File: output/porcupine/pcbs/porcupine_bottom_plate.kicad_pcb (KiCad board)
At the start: 2 copper layers, 129.4 x 113.9 mm, 0 parts

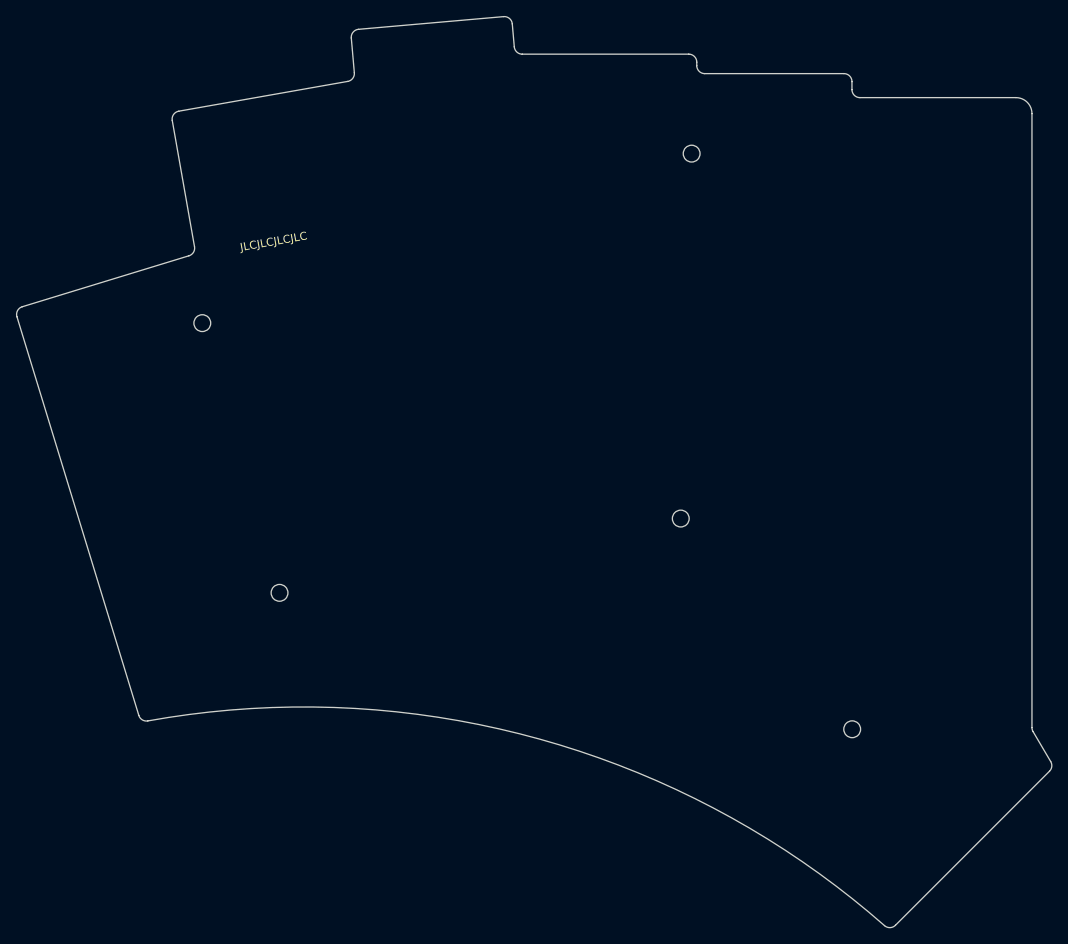
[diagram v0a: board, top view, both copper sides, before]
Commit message: Beschreibung deiner Änderungen
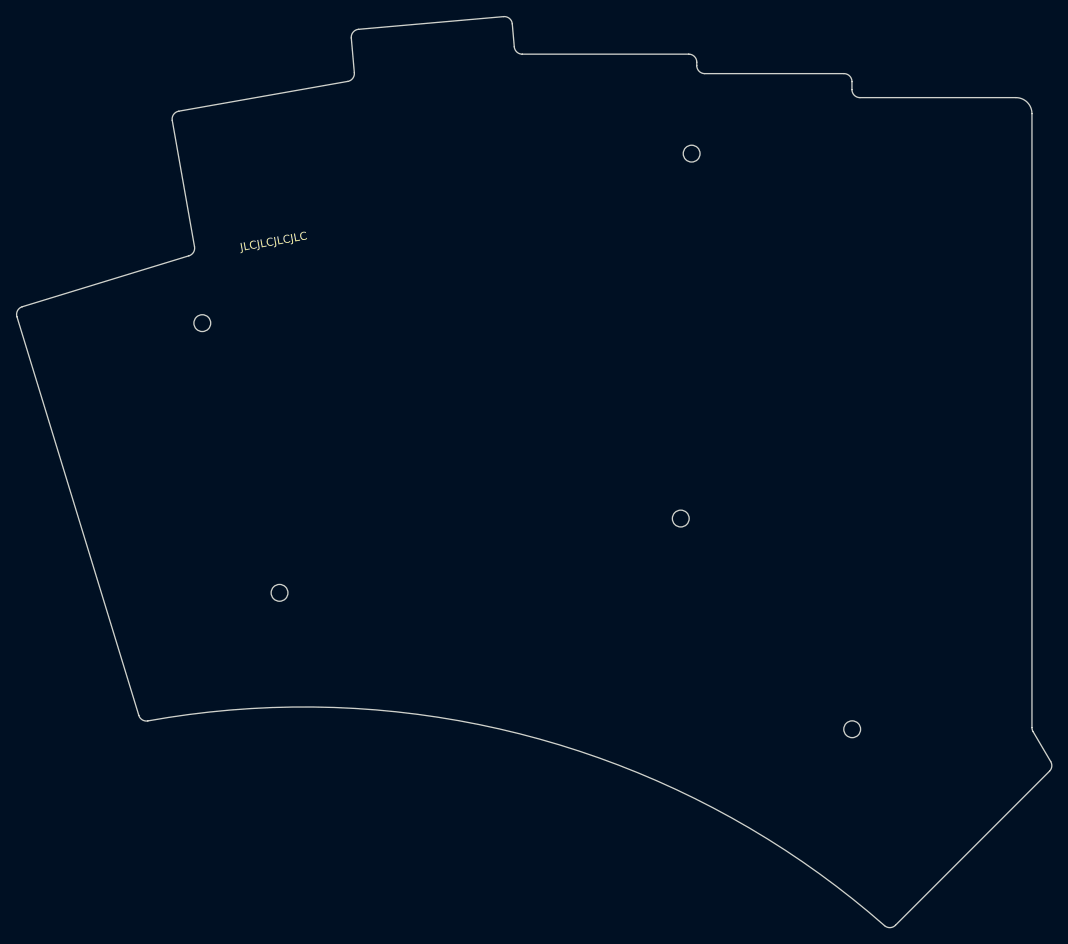
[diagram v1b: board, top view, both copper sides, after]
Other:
- net class Default removed
- net class Power removed
